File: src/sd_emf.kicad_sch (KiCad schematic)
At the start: 10 parts, among them J1 Conn_01x01_Pin, Q1 2N3904, Q2 2N3904, Q3 2N3904, SW1 SW_Push

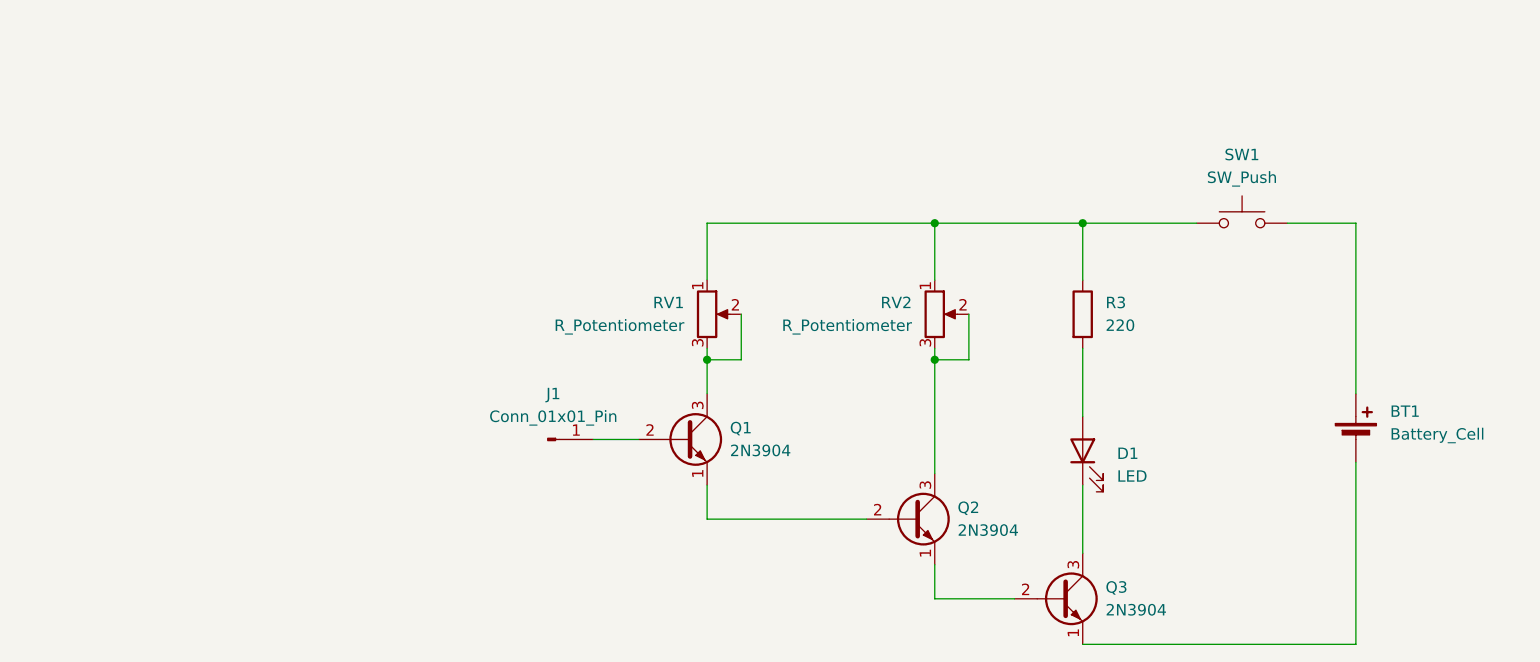
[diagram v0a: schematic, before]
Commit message: docs: update readme, page setup
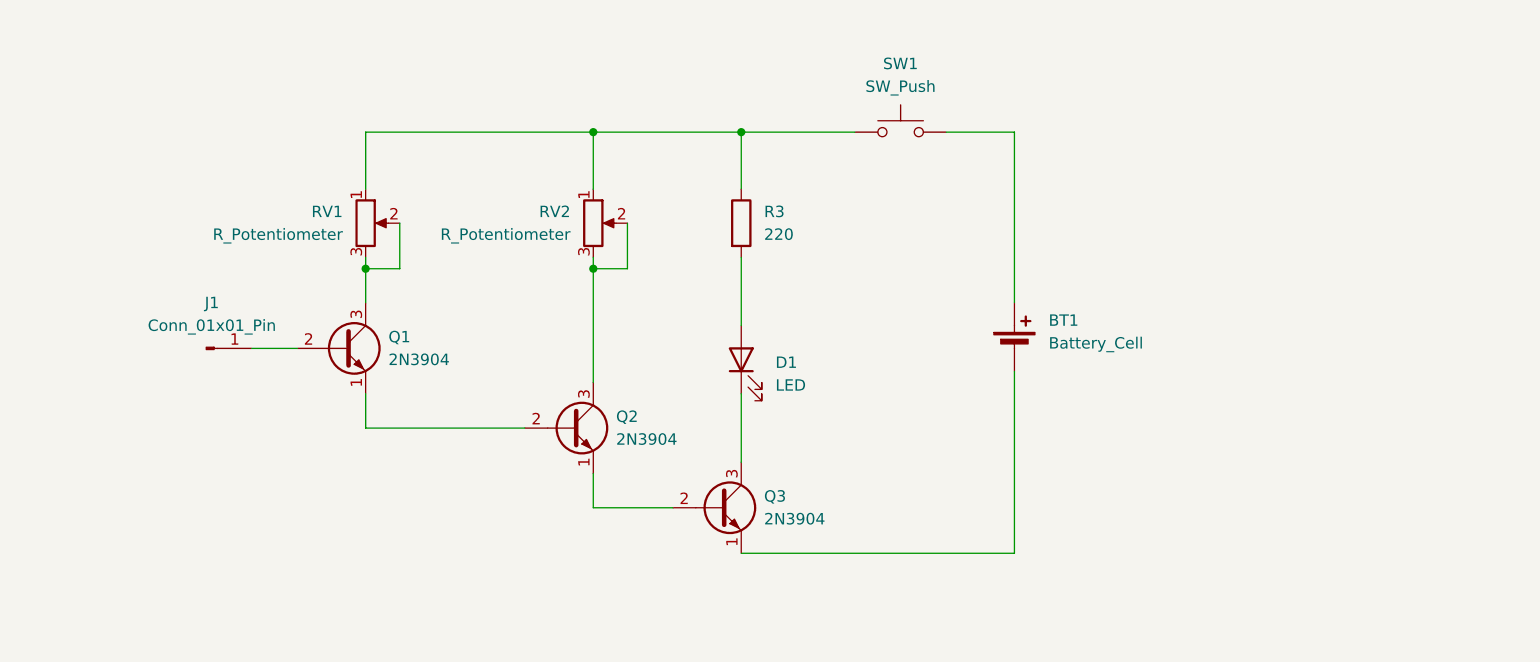
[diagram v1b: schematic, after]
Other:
- moved on the sheet: BT1, D1, J1, Q1, Q2, Q3, R3, RV1, RV2, SW1

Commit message: feat: update pcb
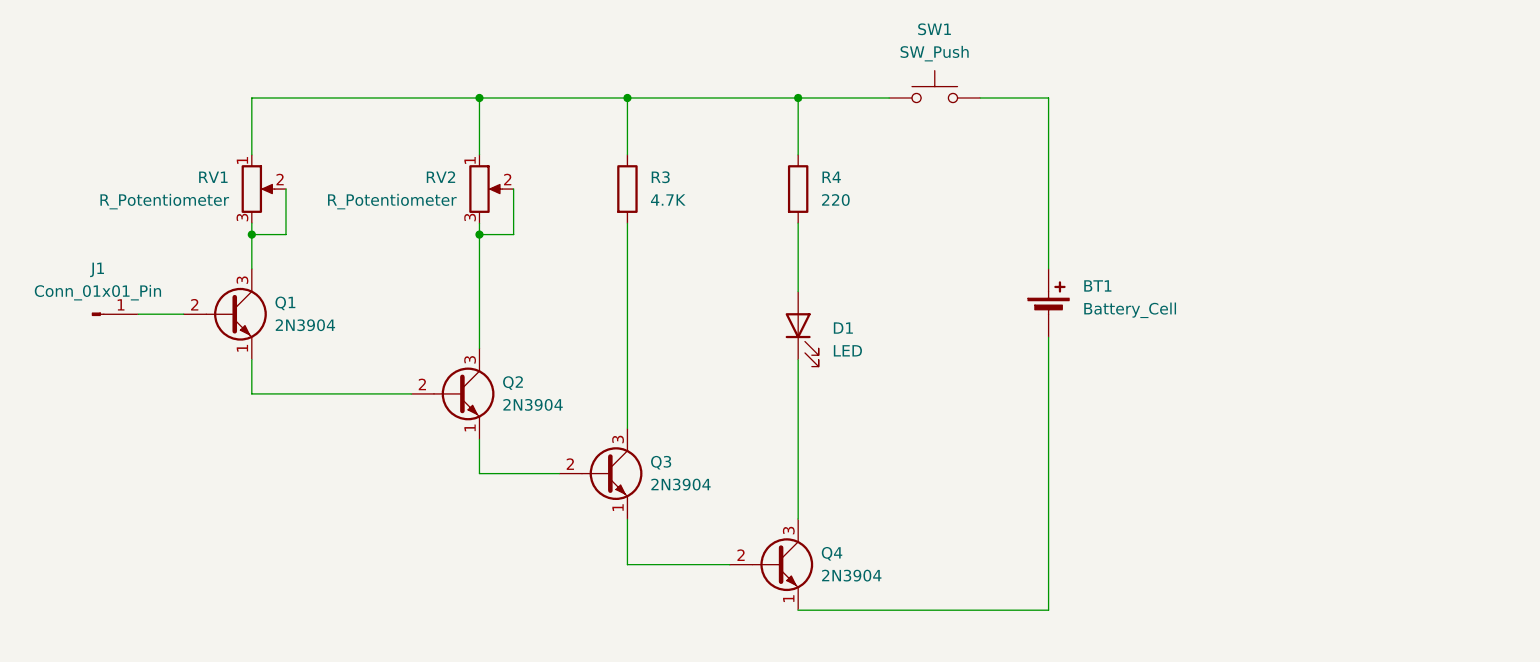
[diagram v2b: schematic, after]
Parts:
- added Q4: 2N3904, Package_TO_SOT_THT:TO-92_HandSolder, symbol Transistor_BJT:2N3904
- added R4: 220, Resistor_THT:R_Axial_DIN0207_L6.3mm_D2.5mm_P7.62mm_Horizontal, symbol Device:R
- R3: value 220 -> 4.7K
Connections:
- net at Q3.1 (E): now also Q4.2 (B); no longer BT1.2 (-)
- net at Q3.3 (C): now also R3.2; no longer D1.1 (K)
- net at R3.1, RV1.1, RV2.1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: now also R4.1
- net at D1.2 (A): now also R4.2; no longer R3.2
- new net: BT1.2 (-), Q4.1 (E)
- new net: D1.1 (K), Q4.3 (C)
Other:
- moved on the sheet: BT1, D1, J1, Q1, Q2, Q3, R3, RV1, RV2, SW1
